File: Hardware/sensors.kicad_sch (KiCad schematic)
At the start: 29 parts, among them IC1 BMP388, J1 Conn_Coaxial, J12 Conn_Coaxial, U13 LSM6DSO, U2 MAX-M10S, U3 74LVC1GU04

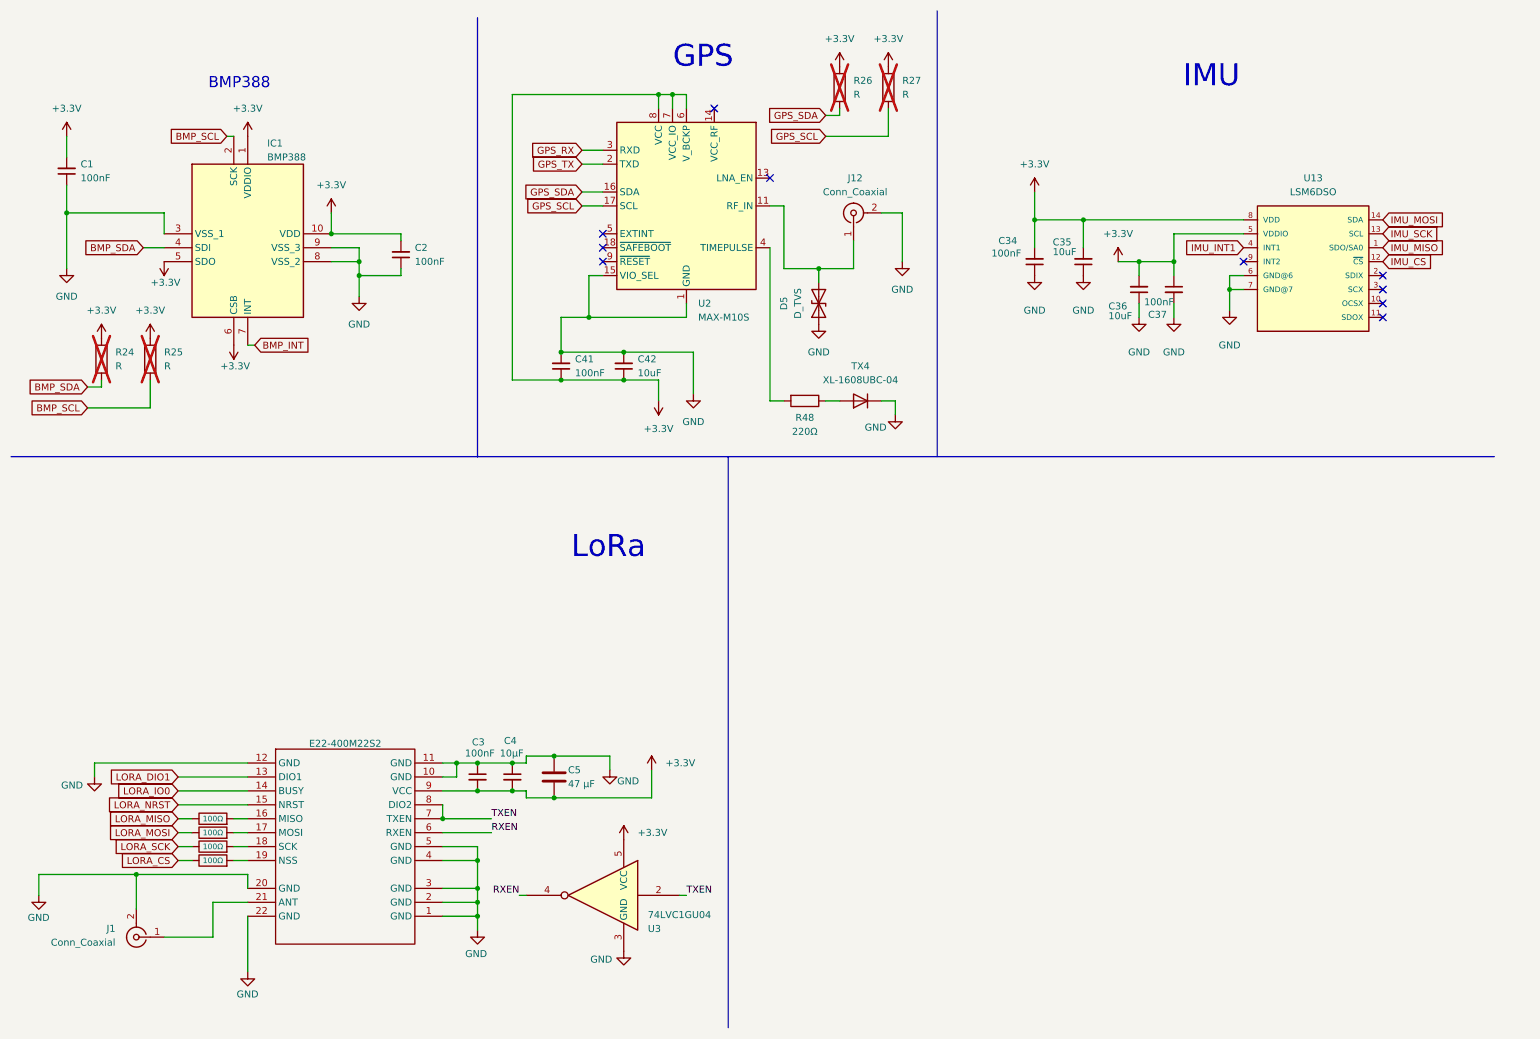
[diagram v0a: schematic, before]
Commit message: Kaut ko palaboju
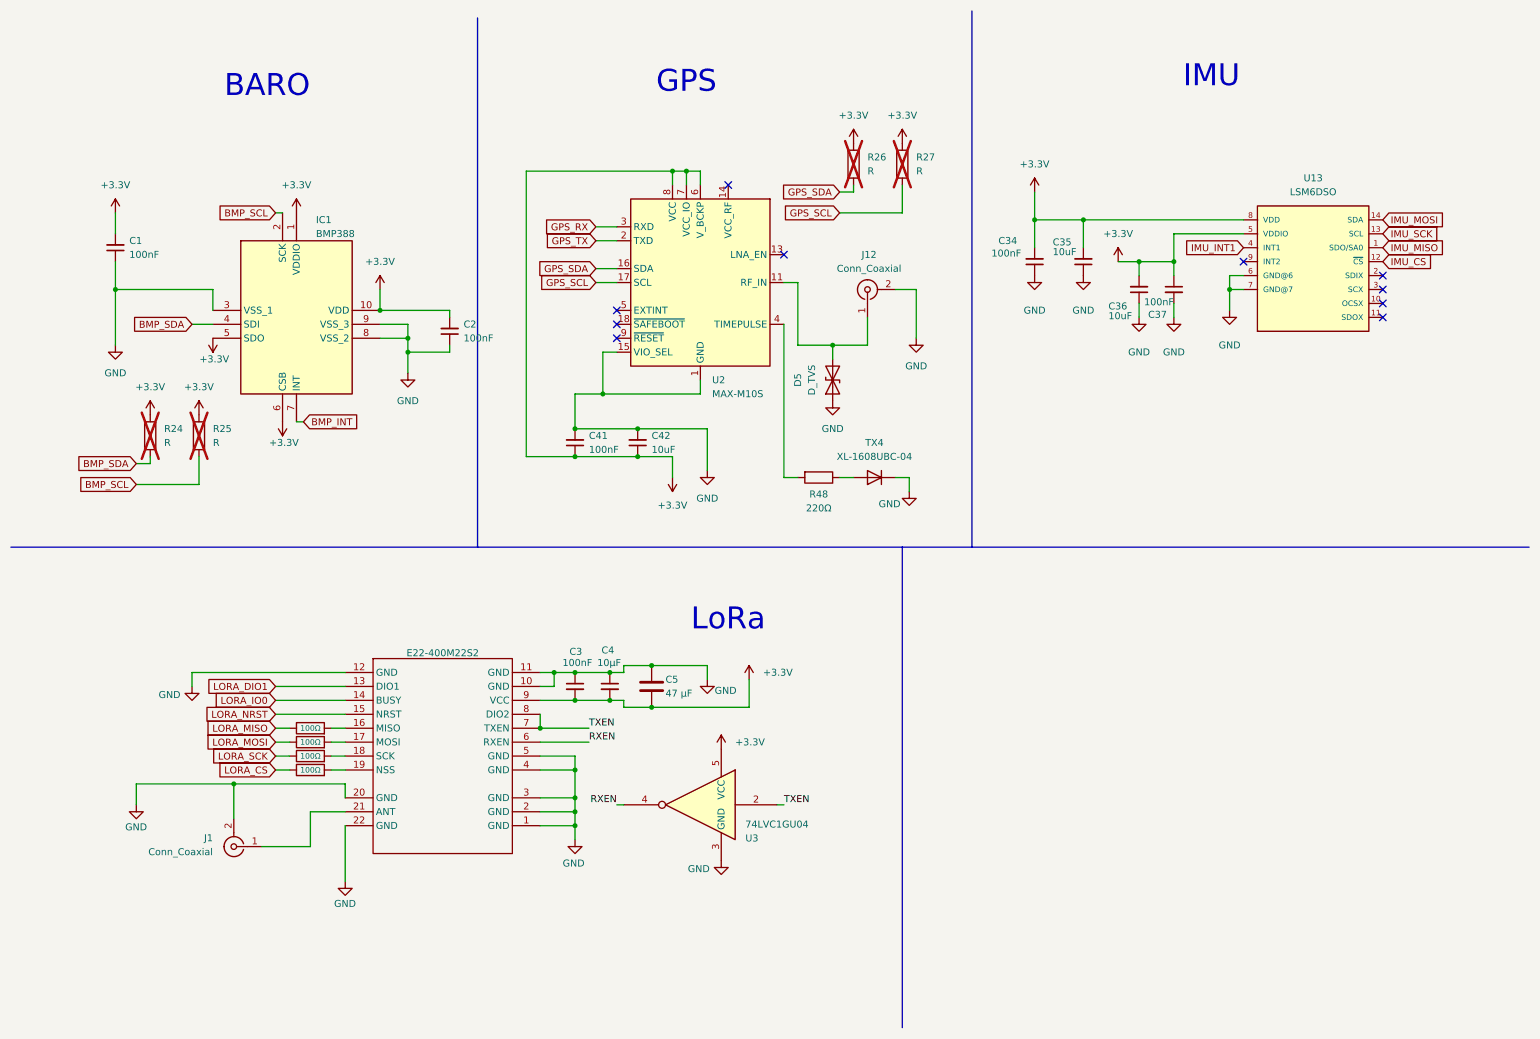
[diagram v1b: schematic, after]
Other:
- note added: "BARO"
- note removed: "BMP388"
- moved on the sheet: C1, C2, C3, C4, C41, C42, C5, D5, E22-400M22S2, IC1, J1, J12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
